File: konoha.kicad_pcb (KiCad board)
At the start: 4 copper layers, 50 x 50 mm, 65 parts, among them J1 Port_1_C, J2 Port_2_C, J3 Port_3, J4 Port_4, J5 Port_Host, J6 Port_Charge_PowerOnly, U1 CH634X, U14 USBLC6-2P6, U15 CH213K, U16 CH217K, U17 CH217K, U18 CH217K, U19 CH217K, Y1 24MHz

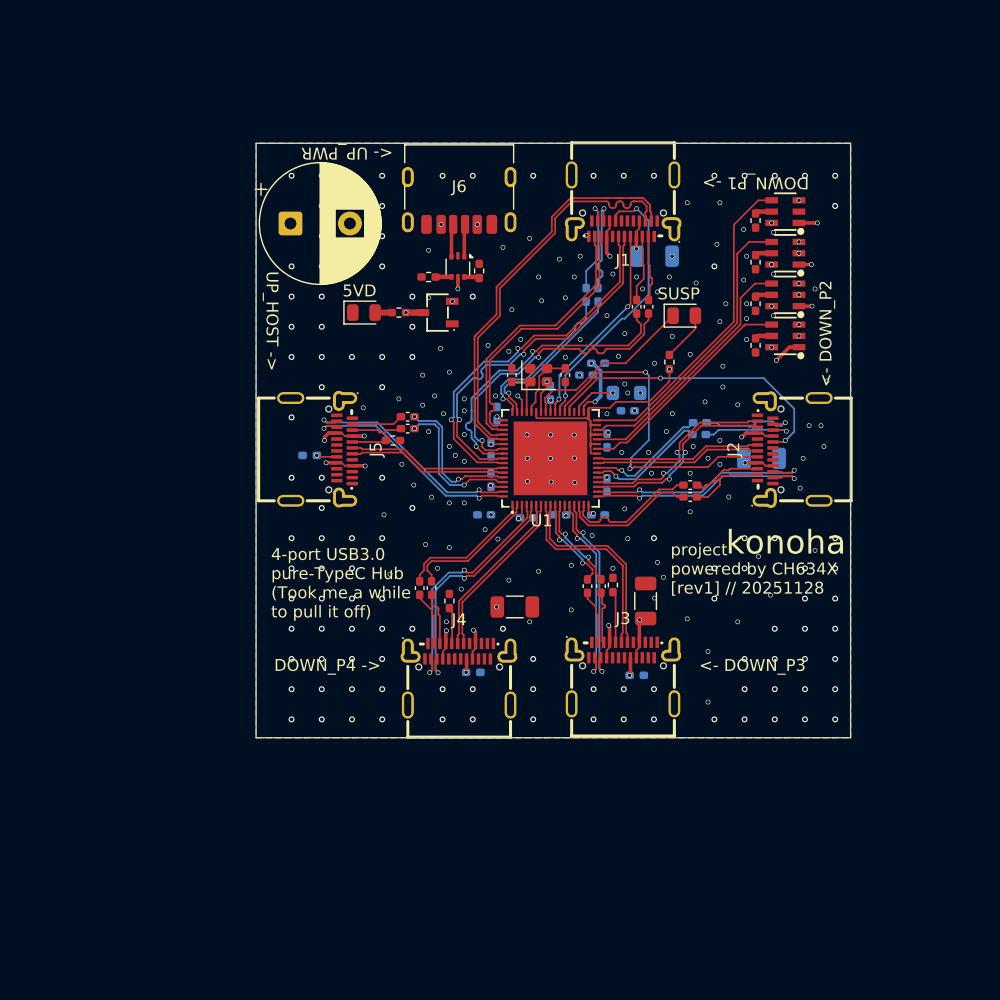
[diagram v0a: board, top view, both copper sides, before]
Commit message: v2 schematic and board
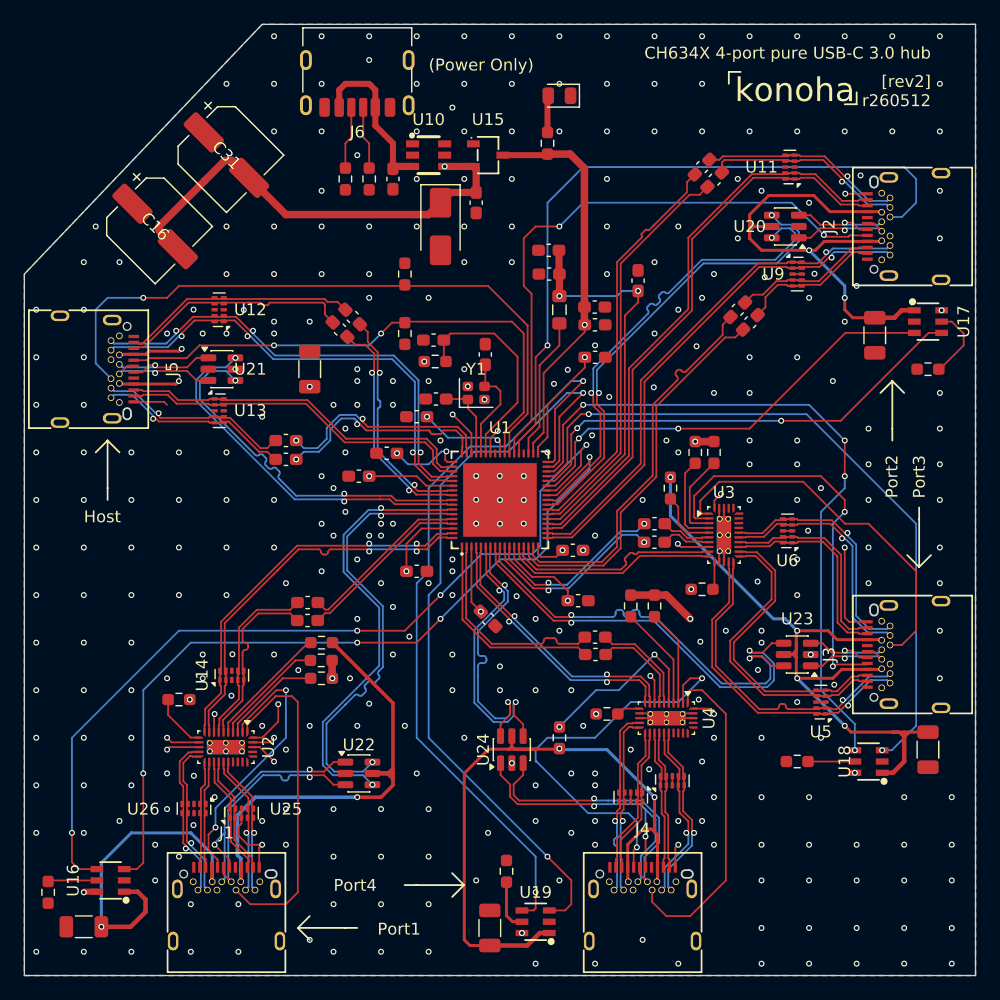
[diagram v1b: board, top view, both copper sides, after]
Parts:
- removed C32, C33, C34: 0.1uF, Capacitor_SMD:C_0402_1005Metric_Pad0.74x0.62mm_HandSolder
- removed D1: SUSP, LED_SMD:LED_0805_2012Metric
- removed R1: 1K, Resistor_SMD:R_0402_1005Metric_Pad0.72x0.64mm_HandSolder
- added C35: 0.1uF, Capacitor_SMD:C_0603_1608Metric_Pad1.08x0.95mm_HandSolder, F.Cu at (103.0, 72.0)
- added C36: 0.1uF, Capacitor_SMD:C_0603_1608Metric_Pad1.08x0.95mm_HandSolder, F.Cu at (103.0, 73.6)
- added C37: 0.1uF, Capacitor_SMD:C_0603_1608Metric_Pad1.08x0.95mm_HandSolder, F.Cu at (98.0, 81.5)
- added C38: 0.1uF, Capacitor_SMD:C_0603_1608Metric_Pad1.08x0.95mm_HandSolder, F.Cu at (98.0, 83.0)
- added C39: 0.1uF, Capacitor_SMD:C_0603_1608Metric_Pad1.08x0.95mm_HandSolder, F.Cu at (73.8, 80.1)
- added C40: 0.1uF, Capacitor_SMD:C_0603_1608Metric_Pad1.08x0.95mm_HandSolder, F.Cu at (73.8, 78.6)
- added C41: 1uF, Capacitor_SMD:C_0603_1608Metric_Pad1.08x0.95mm_HandSolder, F.Cu at (81.0, 43.0)
- added C42: 1uF, Capacitor_SMD:C_0603_1608Metric_Pad1.08x0.95mm_HandSolder, F.Cu at (88.0, 45.0)
- added D3: SMAJ5.0CA, Diode_SMD:D_SMA, F.Cu at (85.0, 47.0)
- added R15: 500K, Resistor_SMD:R_0603_1608Metric_Pad0.98x0.95mm_HandSolder, F.Cu at (108.0, 66.0)
- added R16: 200K, Resistor_SMD:R_0603_1608Metric_Pad0.98x0.95mm_HandSolder, F.Cu at (106.4, 66.0)
- added R17: 200K, Resistor_SMD:R_0603_1608Metric_Pad0.98x0.95mm_HandSolder, F.Cu at (101.0, 78.9)
- added R18: 500K, Resistor_SMD:R_0603_1608Metric_Pad0.98x0.95mm_HandSolder, F.Cu at (103.0, 78.9)
- added R19: 200K, Resistor_SMD:R_0603_1608Metric_Pad0.98x0.95mm_HandSolder, F.Cu at (75.0, 83.5)
- added R20: 500K, Resistor_SMD:R_0603_1608Metric_Pad0.98x0.95mm_HandSolder, F.Cu at (75.0, 85.0)
- added R21: 5.1K, Resistor_SMD:R_0603_1608Metric_Pad0.98x0.95mm_HandSolder, F.Cu at (82.0, 56.0)
- added R22: 5.1K, Resistor_SMD:R_0603_1608Metric_Pad0.98x0.95mm_HandSolder, F.Cu at (82.0, 51.0)
- added R23: 10K, Resistor_SMD:R_0603_1608Metric_Pad0.98x0.95mm_HandSolder, F.Cu at (84.5, 58.4)
- added U10: WS3202E61-6/TR, footprint:SOT-23-6_L2.9-W1.6-P0.95-LS2.8-BR, F.Cu at (84.0, 41.0)
- added U11: TPD4E02B04DQA, Package_SON:USON-10_2.5x1.0mm_P0.5mm, F.Cu at (114.4, 42.0)
- added U12: TPD4E02B04DQA, Package_SON:USON-10_2.5x1.0mm_P0.5mm, F.Cu at (66.4, 54.0)
- added U13: TPD4E02B04DQA, Package_SON:USON-10_2.5x1.0mm_P0.5mm, F.Cu at (66.4, 62.5)
- added U2: HD3SS3220IRNHR, Package_DFN_QFN:Texas_RNH0030A_WQFN-30-1EP_2.5x4.5mm_P0.4mm_EP1.2x3.2mm_ThermalVias, F.Cu at (67.0, 90.8)
- added U20: USBLC6-2SC6, Package_TO_SOT_SMD:SOT-23-6, F.Cu at (114.0, 47.0)
- added U21: USBLC6-2SC6, Package_TO_SOT_SMD:SOT-23-6, F.Cu at (66.6, 59.0)
- added U22: USBLC6-2SC6, Package_TO_SOT_SMD:SOT-23-6, F.Cu at (78.1, 93.0)
- added U23: USBLC6-2SC6, Package_TO_SOT_SMD:SOT-23-6, F.Cu at (115.0, 83.0)
- added U24: USBLC6-2SC6, Package_TO_SOT_SMD:SOT-23-6, F.Cu at (91.0, 91.0)
- added U25: TPD4E02B04DQA, Package_SON:USON-10_2.5x1.0mm_P0.5mm, F.Cu at (64.3, 96.0)
- added U26: TPD4E02B04DQA, Package_SON:USON-10_2.5x1.0mm_P0.5mm, F.Cu at (68.3, 96.3)
- added U3: HD3SS3220IRNHR, Package_DFN_QFN:Texas_RNH0030A_WQFN-30-1EP_2.5x4.5mm_P0.4mm_EP1.2x3.2mm_ThermalVias, F.Cu at (108.8, 72.9)
- added U4: HD3SS3220IRNHR, Package_DFN_QFN:Texas_RNH0030A_WQFN-30-1EP_2.5x4.5mm_P0.4mm_EP1.2x3.2mm_ThermalVias, F.Cu at (104.0, 88.3)
- added U5: TPD4E02B04DQA, Package_SON:USON-10_2.5x1.0mm_P0.5mm, F.Cu at (117.0, 87.0)
- added U6: TPD4E02B04DQA, Package_SON:USON-10_2.5x1.0mm_P0.5mm, F.Cu at (114.2, 72.6)
- added U7: TPD4E02B04DQA, Package_SON:USON-10_2.5x1.0mm_P0.5mm, F.Cu at (101.0, 95.0)
- added U8: TPD4E02B04DQA, Package_SON:USON-10_2.5x1.0mm_P0.5mm, F.Cu at (104.5, 93.6)
- added U9: TPD4E02B04DQA, Package_SON:USON-10_2.5x1.0mm_P0.5mm, F.Cu at (115.0, 51.0)
- C1, C11, C12, C13, C14, C15, C2, C23, C24, C27, C28, C3, C4, C5, C6, C7, C8: footprint Capacitor_SMD:C_0402_1005Metric_Pad0.74x0.62mm_HandSolder -> Capacitor_SMD:C_0603_1608Metric_Pad1.08x0.95mm_HandSolder; moved to F.Cu
- C10, C21, C22, C25, C26, C9: footprint Capacitor_SMD:C_0402_1005Metric_Pad0.74x0.62mm_HandSolder -> Capacitor_SMD:C_0603_1608Metric_Pad1.08x0.95mm_HandSolder
- C16: footprint Capacitor_THT:CP_Radial_D10.0mm_P5.00mm -> Capacitor_SMD:CP_Elec_6.3x7.7
- C17, C18, L1: moved to F.Cu
- C29: value 0.1uF -> 100uF; footprint Capacitor_SMD:C_0402_1005Metric_Pad0.74x0.62mm_HandSolder -> Capacitor_SMD:C_1206_3216Metric
- C30: value 0.1uF -> 100nF; footprint Capacitor_SMD:C_0402_1005Metric_Pad0.74x0.62mm_HandSolder -> Capacitor_SMD:C_0603_1608Metric_Pad1.08x0.95mm_HandSolder
- C31: value 0.1uF -> 470uF; footprint Capacitor_SMD:C_0402_1005Metric_Pad0.74x0.62mm_HandSolder -> Capacitor_SMD:CP_Elec_6.3x7.7
- J1: value Port_1_C -> Port_1; footprint footprint:USB-C-SMD_TYPE-C-24P-QT -> footprint:TYPE-C-USB-SMD_QCHT-143
- J2: value Port_2_C -> Port_2; footprint footprint:USB-C-SMD_TYPE-C-24P-QT -> footprint:TYPE-C-USB-SMD_QCHT-143
- J3, J4, J5: footprint footprint:USB-C-SMD_TYPE-C-24P-QT -> footprint:TYPE-C-USB-SMD_QCHT-143
- R10, R12: value 5.1K -> 200K; footprint Resistor_SMD:R_0402_1005Metric_Pad0.72x0.64mm_HandSolder -> Resistor_SMD:R_0603_1608Metric_Pad0.98x0.95mm_HandSolder; moved to F.Cu
- R11, R9: value 5.1K -> 900K; footprint Resistor_SMD:R_0402_1005Metric_Pad0.72x0.64mm_HandSolder -> Resistor_SMD:R_0603_1608Metric_Pad0.98x0.95mm_HandSolder
- R13: value 56K -> 900K; footprint Resistor_SMD:R_0402_1005Metric_Pad0.72x0.64mm_HandSolder -> Resistor_SMD:R_0603_1608Metric_Pad0.98x0.95mm_HandSolder
- R14: value 56K -> 200K; footprint Resistor_SMD:R_0402_1005Metric_Pad0.72x0.64mm_HandSolder -> Resistor_SMD:R_0603_1608Metric_Pad0.98x0.95mm_HandSolder; moved to F.Cu
- R2, R3, R4: footprint Resistor_SMD:R_0402_1005Metric_Pad0.72x0.64mm_HandSolder -> Resistor_SMD:R_0603_1608Metric_Pad0.98x0.95mm_HandSolder
- R5, R6, R7, R8: value 24K -> 30K; footprint Resistor_SMD:R_0402_1005Metric_Pad0.72x0.64mm_HandSolder -> Resistor_SMD:R_0603_1608Metric_Pad0.98x0.95mm_HandSolder
- U14: value USBLC6-2P6 -> TPD4E02B04DQA; footprint Package_TO_SOT_SMD:SOT-666 -> Package_SON:USON-10_2.5x1.0mm_P0.5mm
- moved R5 75.2 mm to (52.0, 103.0)
- moved U16 72.9 mm to (57.2, 102.0)
- moved J1 67.6 mm to (67.0, 104.0), turned to 0 degrees
- moved U19 63.3 mm to (93.0, 105.5)
- moved R8 58.6 mm to (90.5, 101.2), turned to 90 degrees
- moved C29 52.1 mm to (55.0, 105.9), turned to 180 degrees
- moved U18 43.3 mm to (121.0, 92.0)
- moved R7 42.1 mm to (115.0, 92.0), turned to 180 degrees
- moved C31 40.3 mm to (67.0, 41.0), turned to -45 degrees
- moved U14 39.3 mm to (67.5, 84.8), turned to 90 degrees
- moved C18 38.7 mm to (74.0, 59.0), turned to 90 degrees
- moved C25 34.2 mm to (72.0, 65.0), turned to 0 degrees
- moved C26 34.1 mm to (72.0, 66.6), turned to 0 degrees
- moved C27 31.5 mm to (76.5, 55.7), turned to -45 degrees
- moved C28 30.5 mm to (77.6, 54.6), turned to -45 degrees
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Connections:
- C17 pad 1: VBUS1 -> VBUS2
- C18 pad 1: VBUS2 -> +5VD
- C21 pad 1: Net-(J1-TX1-) -> /P2_SS_AC_TX-
- C21 pad 2: /P1_SS_TX- -> /P2_SS_TX-
- C22 pad 1: Net-(J1-TX1+) -> /P2_SS_AC_TX+
- C22 pad 2: /P1_SS_TX+ -> /P2_SS_TX+
- C23 pad 1: Net-(J1-TX2-) -> /P2C_SS_AC_TX-
- C23 pad 2: /P1C_SS_TX- -> /P2C_SS_TX-
- C24 pad 1: Net-(J1-TX2+) -> /P2C_SS_AC_TX+
- C24 pad 2: /P1C_SS_TX+ -> /P2C_SS_TX+
- C25 pad 1: Net-(J2-TX1-) -> /P1C_SS_AC_TX-
- C25 pad 2: /P2_SS_TX- -> /P1C_SS_TX-
- C26 pad 1: Net-(J2-TX1+) -> /P1C_SS_AC_TX+
- C26 pad 2: /P2_SS_TX+ -> /P1C_SS_TX+
- C27 pad 1: Net-(J2-TX2-) -> /P1_SS_AC_TX-
- C27 pad 2: /P2C_SS_TX- -> /P1_SS_TX-
- C28 pad 1: Net-(J2-TX2+) -> /P1_SS_AC_TX+
- C28 pad 2: /P2C_SS_TX+ -> /P1_SS_TX+
- C29 pad 1: Net-(J3-TX1-) -> VBUS1
- C29 pad 2: /P3_SS_TX- -> GND
- C30 pad 1: Net-(J3-TX1+) -> /RESET
- C30 pad 2: /P3_SS_TX+ -> GND
- C31 pad 1: Net-(J4-TX1-) -> GND
- C31 pad 2: /P4_SS_TX- -> +5V
- J1 pad A10: /P1C_SS_RX- -> /UP_SS_RX2-
- J1 pad A11: /P1C_SS_RX+ -> /UP_SS_RX2+
- J1 pad A2: Net-(J1-TX1+) -> /UP_SS_TX1+
- J1 pad A3: Net-(J1-TX1-) -> /UP_SS_TX1-
- J1 pad A5: /P1_CC1 -> Net-(J1-CC1)
- J1 pad A6: /P1_HS_D+ -> /UP_HS_AC_D+
- J1 pad A7: /P1_HS_D- -> /UP_HS_AC_D-
- J1 pad B10: /P1_SS_RX- -> /UP_SS_RX1-
- J1 pad B11: /P1_SS_RX+ -> /UP_SS_RX1+
- J1 pad B2: Net-(J1-TX2+) -> /UP_SS_TX2+
- J1 pad B3: Net-(J1-TX2-) -> /UP_SS_TX2-
- J1 pad B5: /P1_CC2 -> Net-(J1-CC2)
- J1 pad B6: unconnected-(J1-D+-PadB6) -> /UP_HS_AC_D+
- J1 pad B7: unconnected-(J1-D--PadB7) -> /UP_HS_AC_D-
- J2 pad A2: Net-(J2-TX1+) -> /P2_SS_AC_TX+
- J2 pad A3: Net-(J2-TX1-) -> /P2_SS_AC_TX-
- J2 pad A6: /P2_HS_D+ -> /P2_HS_AC_D+
- J2 pad A7: /P2_HS_D- -> /P2_HS_AC_D-
- J2 pad B2: Net-(J2-TX2+) -> /P2C_SS_AC_TX+
- J2 pad B3: Net-(J2-TX2-) -> /P2C_SS_AC_TX-
- J2 pad B6: unconnected-(J2-D+-PadB6) -> /P2_HS_AC_D+
- J2 pad B7: unconnected-(J2-D--PadB7) -> /P2_HS_AC_D-
- J3 pad A10: unconnected-(J3-RX2--PadA10) -> /P3_SS_RX2-
- J3 pad A11: unconnected-(J3-RX2+-PadA11) -> /P3_SS_RX2+
- J3 pad A2: Net-(J3-TX1+) -> /P3_SS_TX1+
- J3 pad A3: Net-(J3-TX1-) -> /P3_SS_TX1-
- J3 pad A6: /P3_HS_D+ -> /P3_HS_AC_D+
- J3 pad A7: /P3_HS_D- -> /P3_HS_AC_D-
- J3 pad B10: /P3_SS_RX- -> /P3_SS_RX1-
- J3 pad B11: /P3_SS_RX+ -> /P3_SS_RX1+
- J3 pad B2: unconnected-(J3-TX2+-PadB2) -> /P3_SS_TX2+
- J3 pad B3: unconnected-(J3-TX2--PadB3) -> /P3_SS_TX2-
- J3 pad B6: unconnected-(J3-D+-PadB6) -> /P3_HS_AC_D+
- J3 pad B7: unconnected-(J3-D--PadB7) -> /P3_HS_AC_D-
- J4 pad A10: unconnected-(J4-RX2--PadA10) -> /P4_SS_RX2-
- J4 pad A11: unconnected-(J4-RX2+-PadA11) -> /P4_SS_RX2+
- J4 pad A2: Net-(J4-TX1+) -> /P4_SS_TX1+
- J4 pad A3: Net-(J4-TX1-) -> /P4_SS_TX1-
- J4 pad A6: /P4_HS_D+ -> /P4_HS_AC_D+
- J4 pad A7: /P4_HS_D- -> /P4_HS_AC_D-
- J4 pad B10: /P4_SS_RX- -> /P4_SS_RX1-
- J4 pad B11: /P4_SS_RX+ -> /P4_SS_RX1+
- J4 pad B2: unconnected-(J4-TX2+-PadB2) -> /P4_SS_TX2+
- J4 pad B3: unconnected-(J4-TX2--PadB3) -> /P4_SS_TX2-
- J4 pad B6: unconnected-(J4-D+-PadB6) -> /P4_HS_AC_D+
- J4 pad B7: unconnected-(J4-D--PadB7) -> /P4_HS_AC_D-
- J5 pad A10: unconnected-(J5-RX2--PadA10) -> /P1C_SS_RX-
- J5 pad A11: unconnected-(J5-RX2+-PadA11) -> /P1C_SS_RX+
- J5 pad A2: Net-(J5-TX1+) -> /P1_SS_AC_TX+
- J5 pad A3: Net-(J5-TX1-) -> /P1_SS_AC_TX-
- J5 pad A5: Net-(J5-CC1) -> /P1_CC1
- J5 pad A6: /UP_HS_D+ -> /P1_HS_AC_D+
- J5 pad A7: /UP_HS_D- -> /P1_HS_AC_D-
- J5 pad B10: /UP_SS_RX- -> /P1_SS_RX-
- J5 pad B11: /UP_SS_RX+ -> /P1_SS_RX+
- J5 pad B2: unconnected-(J5-TX2+-PadB2) -> /P1C_SS_AC_TX+
- J5 pad B3: unconnected-(J5-TX2--PadB3) -> /P1C_SS_AC_TX-
- J5 pad B5: Net-(J5-CC2) -> /P1_CC2
- J5 pad B6: unconnected-(J5-D+-PadB6) -> /P1_HS_AC_D+
- J5 pad B7: unconnected-(J5-D--PadB7) -> /P1_HS_AC_D-
- J6 pad A9: +5V -> Net-(U10-IN)
- J6 pad B9: +5V -> Net-(U10-IN)
- R10 pad 1: Net-(J3-CC2) -> Net-(U3-DIR)
- R10 pad 2: GND -> +3V3
- R11 pad 1: Net-(J4-CC1) -> Net-(U4-VBUS_DET)
- R11 pad 2: GND -> VBUS4
- R12 pad 1: Net-(J4-CC2) -> Net-(U4-DIR)
- R12 pad 2: GND -> +3V3
- R13 pad 1: Net-(J5-CC1) -> Net-(U2-VBUS_DET)
- R13 pad 2: GND -> VBUS1
- R14 pad 1: Net-(J5-CC2) -> Net-(U2-DIR)
- R14 pad 2: GND -> +3V3
- R3 pad 1: Net-(R3-Pad1) -> Net-(J6-CC1)
- R4 pad 1: Net-(R4-Pad1) -> Net-(J6-CC2)
- R9 pad 1: Net-(J3-CC1) -> Net-(U3-VBUS_DET)
- R9 pad 2: GND -> VBUS3
- U1 pad 1: /P4_SS_TX+ -> /P4_SS_TX-
- U1 pad 10: /P3_SS_TX+ -> /P3_SS_TX-
- U1 pad 11: /P3_SS_TX- -> /P3_SS_TX+
- U1 pad 13: /P3_SS_RX+ -> /P3_SS_RX-
- U1 pad 14: /P3_SS_RX- -> /P3_SS_RX+
- U1 pad 2: /P4_SS_TX- -> /P4_SS_TX+
- U1 pad 27: +3V3 -> /OVCUR_1
- U1 pad 29: +3V3 -> /OVCUR_2
- U1 pad 31: +3V3 -> /OVCUR_3
- U1 pad 33: +3V3 -> /OVCUR_4
- U1 pad 4: /P4_SS_RX+ -> /P4_SS_RX-
- U1 pad 46: +3V3 -> /RESET
- U1 pad 5: /P4_SS_RX- -> /P4_SS_RX+
- U1 pad 55: /P1_SS_RX- -> /P1_SS_RX+
- U1 pad 56: /P1_SS_RX+ -> /P1_SS_RX-
- U1 pad 64: /UP_SS_TX+ -> /UP_SS_TX-
- U1 pad 65: /UP_SS_TX- -> /UP_SS_TX+
- U14 pad 1: Net-(J6-CC1) -> /UP_SS_RX+
- U14 pad 2: GND -> /UP_SS_RX-
- U14 pad 3: Net-(J6-CC2) -> GND
- U14 pad 4: Net-(R4-Pad1) -> /UP_SS_AC_TX-
- U14 pad 5: +5V -> /UP_SS_AC_TX+
- U14 pad 6: Net-(R3-Pad1) -> unconnected-(U14-NC-Pad6)
- U16 pad 3: +3V3 -> /OVCUR_1
- U17 pad 3: +3V3 -> /OVCUR_2
- U18 pad 3: +3V3 -> /OVCUR_3
- U19 pad 3: +3V3 -> /OVCUR_4
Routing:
- net +5V: track 0.95 -> 205.3 mm, vias 8 -> 5
- net +5VD: track 14.1 -> 184.1 mm, vias 8 -> 11
- net +1V2: track 8.64 -> 140.9 mm
- net +3V3: track 23.7 -> 104.4 mm, vias 6 -> 8
- net /OVCUR_1: track 0.00 -> 69.6 mm, vias 0 -> 4
- net /OVCUR_4: track 0.00 -> 65.7 mm, vias 0 -> 2
- net /OVCUR_3: track 0.00 -> 59.5 mm, vias 0 -> 2
- net /PWREN_1: track 19.0 -> 74.7 mm, vias 0 -> 4
- net GND: track 4.84 -> 58.4 mm, vias 247 -> 349
- net VBUS1: track 26.7 -> 72.5 mm, vias 3 -> 2
- net /PWREN_4: track 27.1 -> 66.7 mm, vias 0 -> 2
- net /OVCUR_2: track 0.00 -> 37.4 mm, vias 0 -> 2
- net /P2_CC2: track 25.5 -> 59.4 mm, vias 2 -> 1
- net /PWREN_3: track 24.6 -> 58.6 mm, vias 0 -> 4
- net /P1_CC2: track 23.2 -> 56.3 mm, vias 2 -> 1
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- added copper zone on In2.Cu, net GND
- removed copper zone on In2.Cu, net +1V2
- removed copper zone on In2.Cu, net +3V3
- removed copper zone on In2.Cu, net +5V
- removed copper zone on In2.Cu, net +5VD
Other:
- board size 50 x 50 mm -> 80 x 80 mm
- board text added: "(Power Only)"
- board text added: "CH634X 4-port pure USB-C 3.0 hub"
- board text added: "Host"
- board text added: "Port1"
- board text added: "Port2"
- board text added: "Port3"
- board text added: "Port4"
- board text added: "[rev2] r260512"
- board text removed: "4-port USB3.0 pure-TypeC Hub (Took me a while to pull it off)"
- board text removed: "5VD"
- board text removed: "<- DOWN_P2"
- board text removed: "<- DOWN_P3"
- board text removed: "<- UP_PWR"
- board text removed: "DOWN_P1 ->"
- board text removed: "DOWN_P4 ->"
- board text removed: "SUSP"
- board text removed: "UP_HOST ->"
- board text removed: "project powered by CH634X [rev1] // 20251128"
